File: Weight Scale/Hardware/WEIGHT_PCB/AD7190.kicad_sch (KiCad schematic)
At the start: 46 parts, among them IC1 AD7190BRUZ

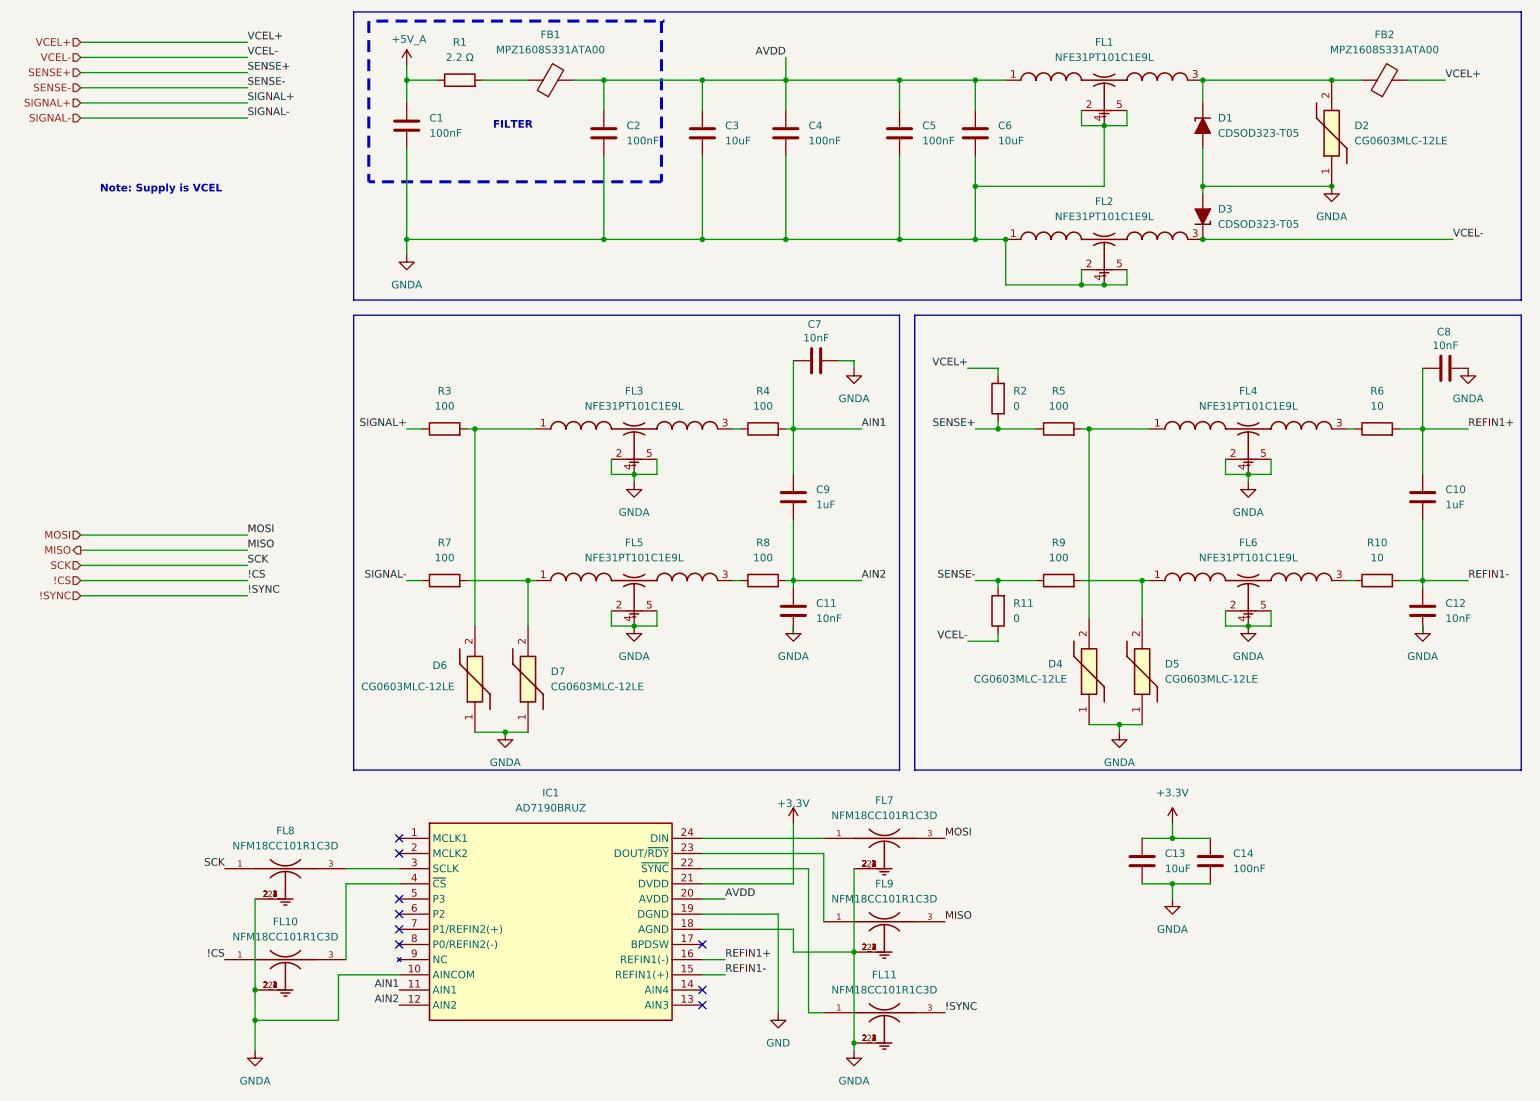
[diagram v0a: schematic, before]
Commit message: update schematics
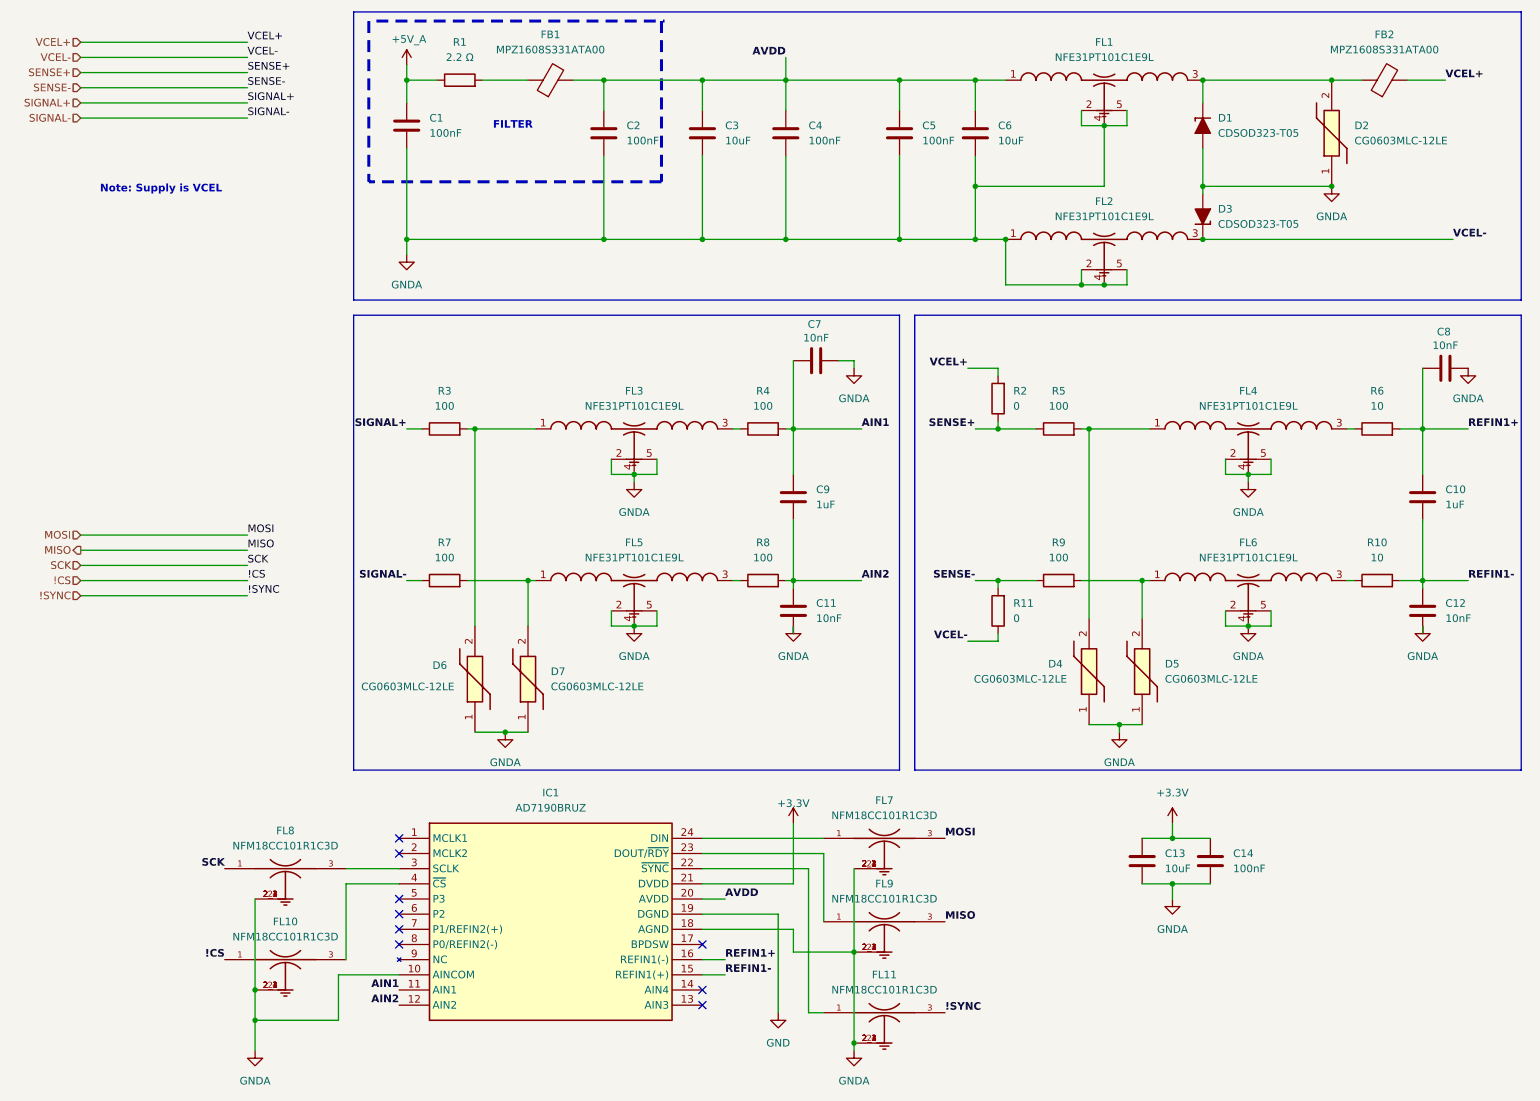
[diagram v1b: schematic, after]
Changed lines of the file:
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@@
 			(font
 				(size 1.27 1.27)
+				(bold yes)
 			)
 			(justify left bottom)
@@
 				(size 1.27 1.27)
 				(thickness 0.1588)
+				(bold yes)
 			)
 			(justify right bottom)
@@
 				(size 1.27 1.27)
 				(thickness 0.1588)
+				(bold yes)
 			)
 			(justify right bottom)
@@
 				(size 1.27 1.27)
 				(thickness 0.1588)
+				(bold yes)
 			)
 			(justify left bottom)
@@
 				(size 1.27 1.27)
 				(thickness 0.1588)
+				(bold yes)
 			)
 			(justify left bottom)
@@
 				(size 1.27 1.27)
 				(thickness 0.1588)
+				(bold yes)
 			)
 			(justify left bottom)
@@
 			(font
 				(size 1.27 1.27)
+				(bold yes)
 			)
 			(justify right bottom)
@@
 				(size 1.27 1.27)
 				(thickness 0.1588)
+				(bold yes)
 			)
 			(justify right bottom)
@@
 				(size 1.27 1.27)
 				(thickness 0.1588)
+				(bold yes)
 			)
 			(justify right bottom)
@@
 				(size 1.27 1.27)
 				(thickness 0.1588)
+				(bold yes)
 			)
 			(justify right bottom)
@@
 			(font
 				(size 1.27 1.27)
+				(bold yes)
 			)
 			(justify left bottom)
@@
 				(size 1.27 1.27)
 				(thickness 0.1588)
+				(bold yes)
 			)
 			(justify left bottom)
@@
 				(size 1.27 1.27)
 				(thickness 0.1588)
+				(bold yes)
 			)
 			(justify left bottom)
@@
 			(font
 				(size 1.27 1.27)
+				(bold yes)
 			)
 			(justify left bottom)
@@
 				(size 1.27 1.27)
 				(thickness 0.1588)
+				(bold yes)
 			)
 			(justify left bottom)
@@
 				(size 1.27 1.27)
 				(thickness 0.1588)
+				(bold yes)
 			)
 			(justify left bottom)
@@
 				(size 1.27 1.27)
 				(thickness 0.1588)
+				(bold yes)
 			)
 			(justify left bottom)
@@
 				(size 1.27 1.27)
 				(thickness 0.1588)
+				(bold yes)
 			)
 			(justify right bottom)
@@
 				(size 1.27 1.27)
 				(thickness 0.1588)
+				(bold yes)
 			)
 			(justify right bottom)
@@
 				(size 1.27 1.27)
 				(thickness 0.1588)
+				(bold yes)
 			)
 			(justify right bottom)
@@
 				(size 1.27 1.27)
 				(thickness 0.1588)
+				(bold yes)
 			)
 			(justify right bottom)
@@
 			(font
 				(size 1.27 1.27)
+				(bold yes)
 			)
 			(justify right bottom)
@@
 				(size 1.27 1.27)
 				(thickness 0.1588)
-			)
-			(justify left bottom)
+				(bold yes)
+			)
+			(justify left bottom)
